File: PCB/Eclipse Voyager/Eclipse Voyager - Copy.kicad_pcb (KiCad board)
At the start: 2 copper layers, 75 x 85 mm, 153 parts, among them J1 Conn_01x04_Male, U1 TPD4E05U06DQAR

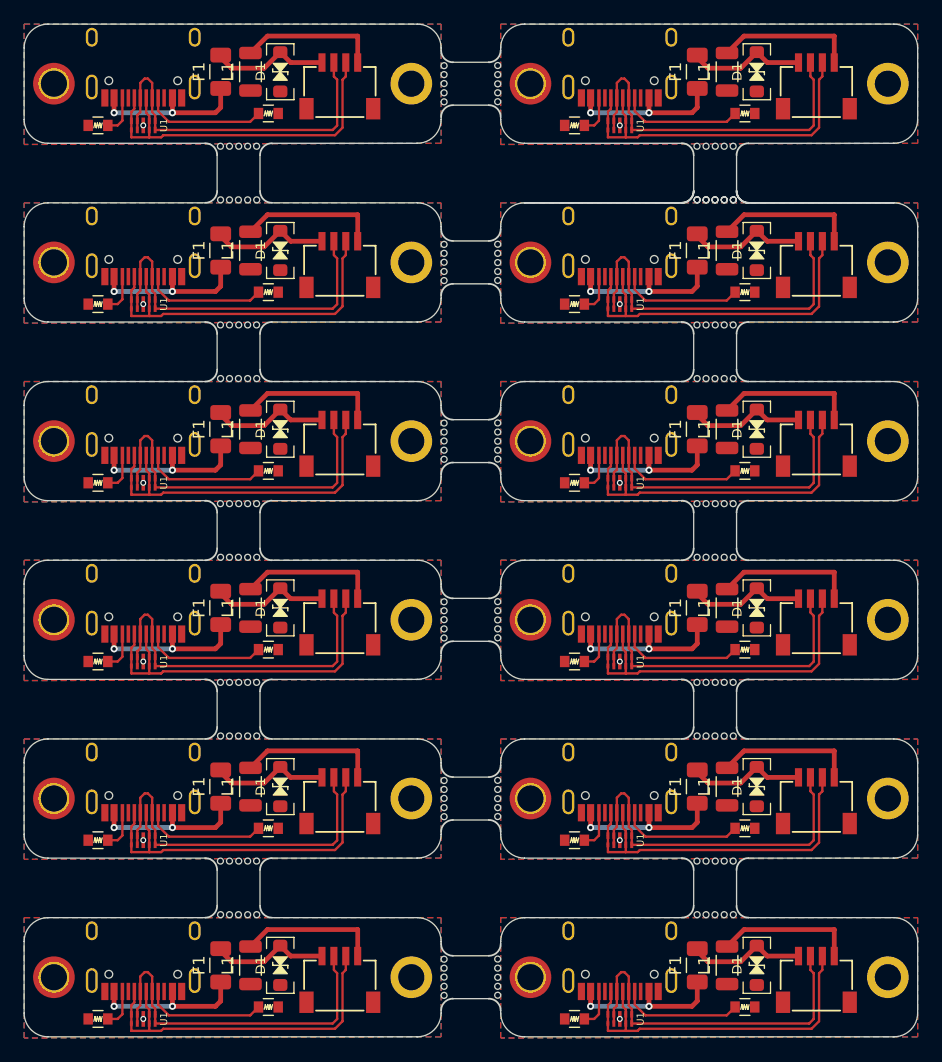
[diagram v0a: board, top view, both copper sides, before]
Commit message: PCB update
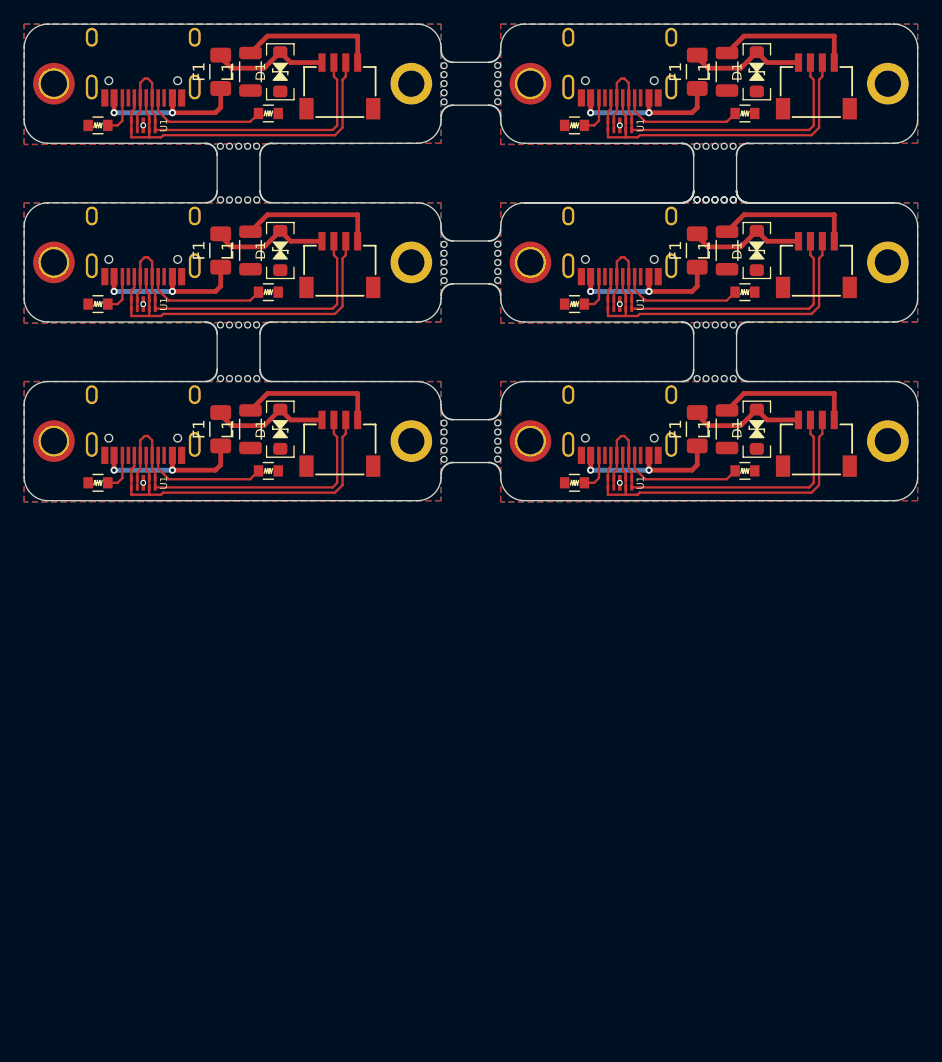
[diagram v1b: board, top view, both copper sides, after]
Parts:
- removed the D1 at (183.5, 105.5)
- removed the D1 at (143.5, 105.5)
- removed the D1 at (183.5, 90.5)
- removed the D1 at (143.5, 90.5)
- removed the D1 at (183.5, 75.5)
- removed the D1 at (143.5, 75.5)
- removed the F1 at (178.5, 105.5)
- removed the F1 at (138.5, 105.5)
- removed the F1 at (178.5, 90.5)
- removed the F1 at (138.5, 90.5)
- removed the F1 at (178.5, 75.5)
- removed the F1 at (138.5, 75.5)
- removed the H1 at (194.5, 106.5)
- removed the H1 at (154.5, 106.5)
- removed the H1 at (194.5, 91.5)
- removed the H1 at (154.5, 91.5)
- removed the H1 at (194.5, 76.5)
- removed the H1 at (154.5, 76.5)
- removed the H2 at (164.5, 106.5)
- removed the H2 at (124.5, 106.5)
- removed the H2 at (164.5, 91.5)
- removed the H2 at (124.5, 91.5)
- removed the H2 at (164.5, 76.5)
- removed the H2 at (124.5, 76.5)
- removed the J1 at (188.5, 109.5)
- removed the J1 at (148.5, 109.5)
- removed the J1 at (188.5, 94.5)
- removed the J1 at (148.5, 94.5)
- removed the J1 at (188.5, 79.5)
- removed the J1 at (148.5, 79.5)
- removed the L1 at (181.0, 105.5)
- removed the L1 at (141.0, 105.5)
- removed the L1 at (181.0, 90.5)
- removed the L1 at (141.0, 90.5)
- removed the L1 at (181.0, 75.5)
- removed the L1 at (141.0, 75.5)
- removed the R1 at (182.5, 109.0)
- removed the R1 at (142.5, 109.0)
- removed the R1 at (182.5, 94.0)
- removed the R1 at (142.5, 94.0)
- removed the R1 at (182.5, 79.0)
- removed the R1 at (142.5, 79.0)
- removed the R2 at (168.2, 110.0)
- removed the R2 at (128.2, 110.0)
- removed the R2 at (168.2, 95.0)
- removed the R2 at (128.2, 95.0)
- removed the R2 at (168.2, 80.0)
- removed the R2 at (128.2, 80.0)
- removed the U1 at (172.0, 110.0)
- removed the U1 at (132.0, 110.0)
- removed the U1 at (172.0, 95.0)
- removed the U1 at (132.0, 95.0)
- removed the U1 at (172.0, 80.0)
- removed the U1 at (132.0, 80.0)
- removed the USB1 at (172.0, 100.0)
- removed the USB1 at (132.0, 100.0)
- removed the USB1 at (172.0, 85.0)
- removed the USB1 at (132.0, 85.0)
- removed the USB1 at (172.0, 70.0)
- removed the USB1 at (132.0, 70.0)
- removed the mouse-bite-3mm-slot at (180.0, 100.5)
- removed the mouse-bite-3mm-slot at (140.0, 100.5)
- removed the mouse-bite-3mm-slot at (180.0, 85.5)
- removed the mouse-bite-3mm-slot at (140.0, 85.5)
- removed the mouse-bite-3mm-slot at (180.0, 70.5)
- removed the mouse-bite-3mm-slot at (140.0, 70.5)
- removed the mouse-bite-3mm-slot at (180.0, 97.5)
- removed the mouse-bite-3mm-slot at (158.0, 106.5)
- removed the mouse-bite-3mm-slot at (158.0, 91.5)
- removed the mouse-bite-3mm-slot at (158.0, 76.5)
- removed the mouse-bite-3mm-slot at (161.0, 106.5)
- removed the mouse-bite-3mm-slot at (161.0, 91.5)
- removed the mouse-bite-3mm-slot at (161.0, 76.5)
- removed the mouse-bite-3mm-slot at (140.0, 97.5)
- removed the mouse-bite-3mm-slot at (180.0, 82.5)
- removed the mouse-bite-3mm-slot at (140.0, 82.5)
- removed the mouse-bite-3mm-slot at (180.0, 67.5)
- removed the mouse-bite-3mm-slot at (140.0, 67.5)
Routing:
- net D+: track 365.5 -> 182.8 mm
- net D-: track 362.8 -> 181.4 mm
- net VBUS: track 161.1 -> 80.5 mm, vias 24 -> 12
- net GND: track 141.8 -> 70.9 mm
- net Net-(R1-Pad2): track 122.3 -> 61.2 mm
- net +5V: track 117.5 -> 58.8 mm
- net Net-(R2-Pad2): track 39.5 -> 19.8 mm
- net GNDPWR: track 9.24 -> 4.62 mm, vias 12 -> 6
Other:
- board size 75 x 85 mm -> 75 x 40 mm
